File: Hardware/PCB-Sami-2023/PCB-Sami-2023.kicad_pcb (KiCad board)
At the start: 2 copper layers, 75 x 40.2 mm, 44 parts, among them J10 Bateria, J9 STEP_DOWN, P1 TatamiDerecho, P2 TatamiIzquierdo, P3 SharpDerecho, P4 SharpIzquierdo, P5 LDR, P6 MotorIzquierdo, P7 MotorDerecho, P8 Pantalla Oled, U1 ESP32-DEVKIT-V1

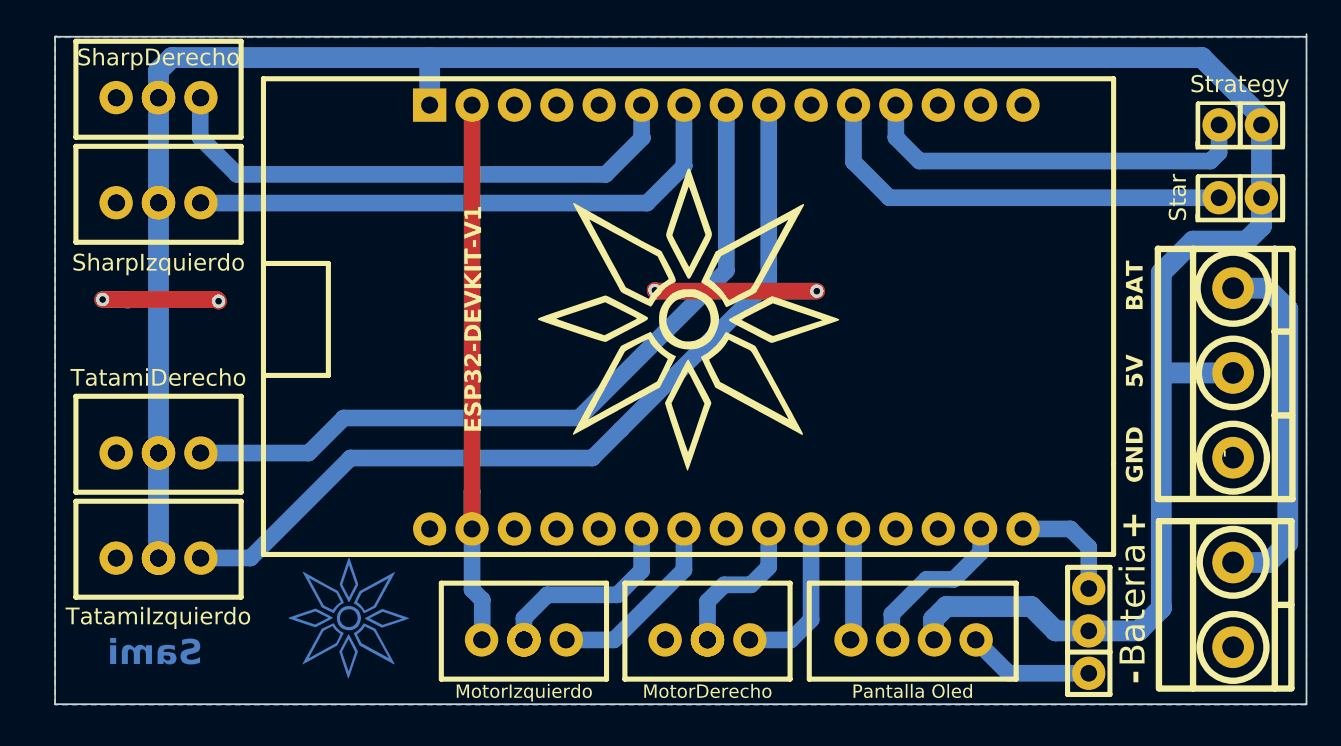
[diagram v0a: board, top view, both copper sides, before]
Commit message: agregue ultimos detalles
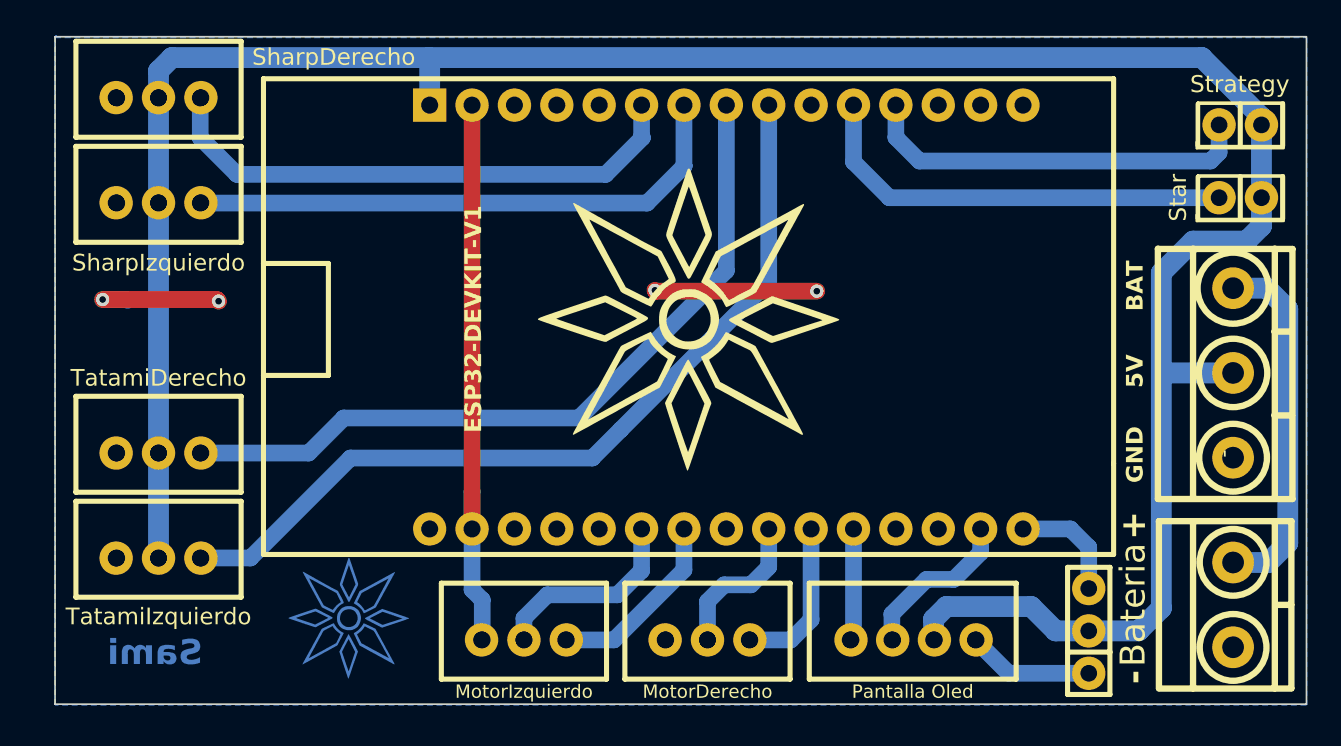
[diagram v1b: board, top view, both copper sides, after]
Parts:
- removed the ? at (113.1, 61.6)
- removed the ? at (113.1, 76.6)
- removed the ? at (113.1, 82.9)
- removed the ? at (135.0, 87.8)
- removed the ? at (113.1, 55.3)
- removed the ? at (146.0, 87.8)
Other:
- board size 75 x 40.2 mm -> 75 x 40 mm
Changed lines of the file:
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@@
     (pad_to_mask_clearance 0)
     (pcbplotparams
-      (layerselection 0x0000010_7ffffffe)
+      (layerselection 0x0000020_7ffffffe)
       (plot_on_all_layers_selection 0x0001000_00000000)
       (disableapertmacros false)
@@
         (effects (font (size 1.27 1.27) (thickness 0.15)))
     )
-    (pad "1" thru_hole circle (at 0 0 180) (size 2 2) (drill 1.00076) (layers "*.Cu" "*.Mask" "F.SilkS")
-      (net 2 "+5V") (pinfunction "1") (pintype "passive"))
-  )
-  (footprint "" (layer "F.Cu")
-    (at 113.1 76.6)
-    (fp_text reference "" (at 0 0) (layer "F.SilkS")
-        (effects (font (size 1.27 1.27) (thickness 0.15)))
-    )
-    (fp_text value "" (at 0 0) (layer "F.SilkS")
-        (effects (font (size 1.27 1.27) (thickness 0.15)))
-    )
     (pad "2" thru_hole circle (at 0 0 180) (size 2 2) (drill 1.00076) (layers "*.Cu" "*.Mask" "F.SilkS")
       (net 6 "/START") (pinfunction "2") (pintype "passive"))
   )
-  (footprint "" (layer "F.Cu")
-    (at 135 87.8)
-    (fp_text reference "" (at 0 0) (layer "F.SilkS")
-        (effects (font (size 1.27 1.27) (thickness 0.15)))
-    )
-    (fp_text value "" (at 0 0) (layer "F.SilkS")
-        (effects (font (size 1.27 1.27) (thickness 0.15)))
-    )
-    (pad "1" thru_hole circle (at 0 0 180) (size 2 2) (drill 1.00076) (layers "*.Cu" "*.Mask" "F.SilkS")
-      (net 2 "+5V") (pinfunction "1") (pintype "passive"))
-  )
-  (footprint "" (layer "F.Cu")
-    (at 113.1 55.3)
-    (fp_text reference "" (at 0 0) (layer "F.SilkS")
-        (effects (font (size 1.27 1.27) (thickness 0.15)))
-    )
-    (fp_text value "" (at 0 0) (layer "F.SilkS")
-        (effects (font (size 1.27 1.27) (thickness 0.15)))
-    )
-    (pad "1" thru_hole circle (at 0 0 180) (size 2 2) (drill 1.00076) (layers "*.Cu" "*.Mask" "F.SilkS")
-      (net 2 "+5V") (pinfunction "1") (pintype "passive"))
-  )
-  (footprint "" (layer "F.Cu")
-    (at 146 87.8)
-    (fp_text reference "" (at 0 0) (layer "F.SilkS")
-        (effects (font (size 1.27 1.27) (thickness 0.15)))
-    )
-    (fp_text value "" (at 0 0) (layer "F.SilkS")
-        (effects (font (size 1.27 1.27) (thickness 0.15)))
-    )
-    (pad "1" thru_hole circle (at 0 0 180) (size 2 2) (drill 1.00076) (layers "*.Cu" "*.Mask" "F.SilkS")
-      (net 2 "+5V") (pinfunction "1") (pintype "passive"))
-  )
   (footprint "EESTN5:Pin_Header_2" (layer "F.Cu")
     (at 177.93 57.2525 180)
@@
       (stroke (width 0) (type solid)) (fill solid) (layer "B.Cu"))
   )
-  (footprint "" (layer "F.Cu")
-    (at 113.1 61.6)
-    (fp_text reference "" (at 0 0) (layer "F.SilkS")
-        (effects (font (size 1.27 1.27) (thickness 0.15)))
-    )
-    (fp_text value "" (at 0 0) (layer "F.SilkS")
-        (effects (font (size 1.27 1.27) (thickness 0.15)))
-    )
-    (pad "1" thru_hole circle (at 0 0 180) (size 2 2) (drill 1.00076) (layers "*.Cu" "*.Mask" "F.SilkS")
-      (net 2 "+5V") (pinfunction "1") (pintype "passive"))
-  )
   (footprint "EESTN5:Pin_Header_2" (layer "F.Cu")
     (at 177.93 61.6175 180)
@@
       (net 6 "/START") (pinfunction "2") (pintype "passive"))
   )
-  (footprint "" (layer "F.Cu")
-    (at 113.1 82.9)
-    (fp_text reference "" (at 0 0) (layer "F.SilkS")
-        (effects (font (size 1.27 1.27) (thickness 0.15)))
-    )
-    (fp_text value "" (at 0 0) (layer "F.SilkS")
-        (effects (font (size 1.27 1.27) (thickness 0.15)))
-    )
-    (pad "1" thru_hole circle (at 0 0 180) (size 2 2) (drill 1.00076) (layers "*.Cu" "*.Mask" "F.SilkS")
-      (net 2 "+5V") (pinfunction "1") (pintype "passive"))
-  )
   (footprint "footprints:JstXH4P" (layer "F.Cu")
     (at 158.3 87.275)
@@
         (effects (font (size 1 1) (thickness 0.15)))
     )
-    (fp_text value "SharpDerecho" (at 0 -1.9) (layer "F.SilkS")
+    (fp_text value "SharpDerecho" (at 10.5 -1.93) (layer "F.SilkS")
         (effects (font (size 1 1) (thickness 0.15)))
     )
@@
   (gr_line (start 106.9 51.65) (end 106.9 91.65)
     (stroke (width 0.1) (type default)) (layer "Edge.Cuts"))
-  (gr_line (start 181.9 91.65) (end 181.9 51.5)
+  (gr_line (start 181.9 91.65) (end 181.9 51.7)
     (stroke (width 0.1) (type default)) (layer "Edge.Cuts"))
   (gr_line (start 181.9 51.65) (end 106.9 51.65)
